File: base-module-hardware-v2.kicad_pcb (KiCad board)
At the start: 4 copper layers, 99.7 x 99.7 mm, 270 parts, among them K1 CONN_3, P1 PINBALL-CONNECTOR, P2 PINBALL-CONNECTOR, P3 SOLENOID-CONNECTOR, P4 CONN_16, P5 CONN_16, P6 HE10-34, Q1 BC846, Q10 DMN6040SSD, Q11 BC846, Q12 BC846, Q13 DMP2240UDM, Q14 DMP2240UDM, Q15 BC846, Q16 BC846, Q17 BC846, Q18 BC846, Q19 DMN6040SSD, Q2 BC846, Q20 DMN6040SSD, Q21 BC846, Q22 BC846, Q23 BC846, Q24 BC846, Q25 BC846, Q26 BC846, Q27 BC846, Q28 BC846, Q3 DMN6040SSD, Q30 FDD5614P, Q31 BC846, Q32 BSS138, Q4 DMN6040SSD, Q5 BC846, Q6 BC846, Q7 BC846, Q8 BC846, Q9 DMN6040SSD, U1 74LVC14, U2 STM32F072R, U3 MCP2562, U4 MC78L05, U5 AP1117IE33G, U6 ZXCT1086E5TA, U7 ZXCT1107SA-7, U8 LM7805CT, U9 MMA8653FC, X1 8.000 MHz

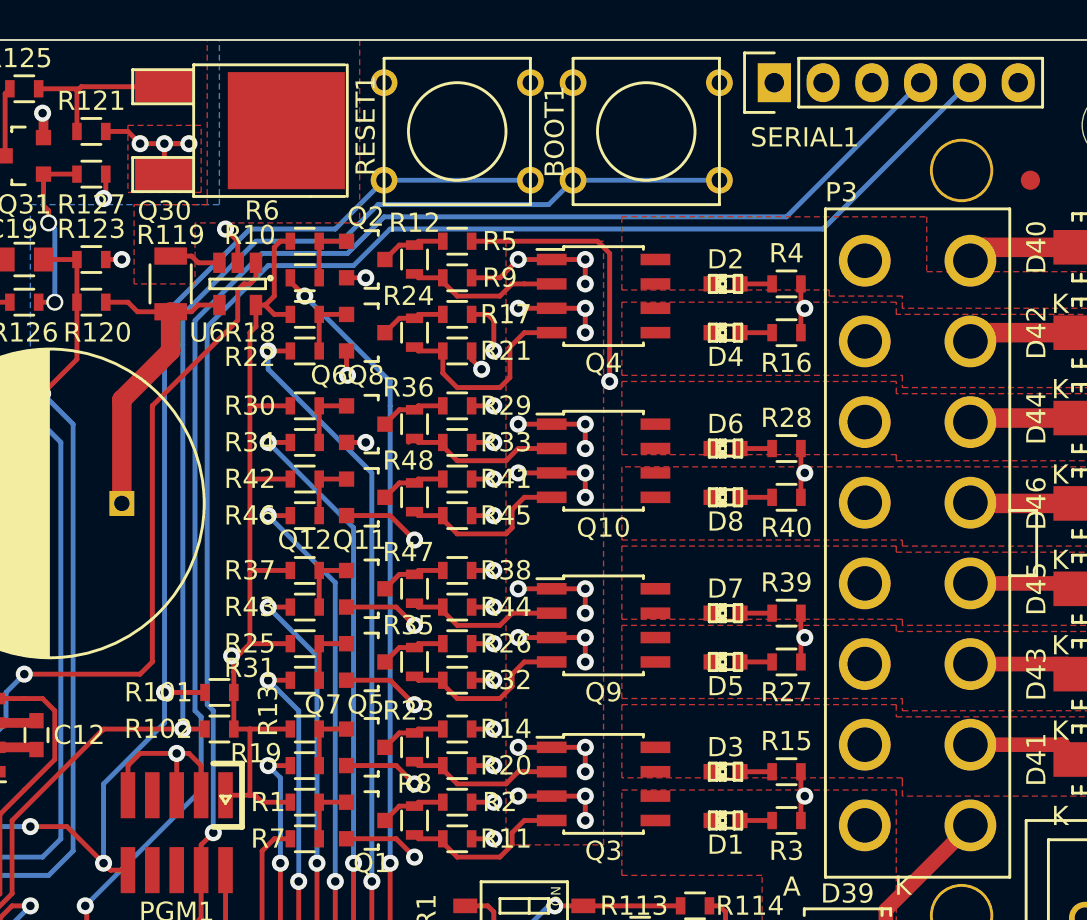
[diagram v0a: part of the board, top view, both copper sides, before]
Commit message: Latest changes (so old I don't remember)
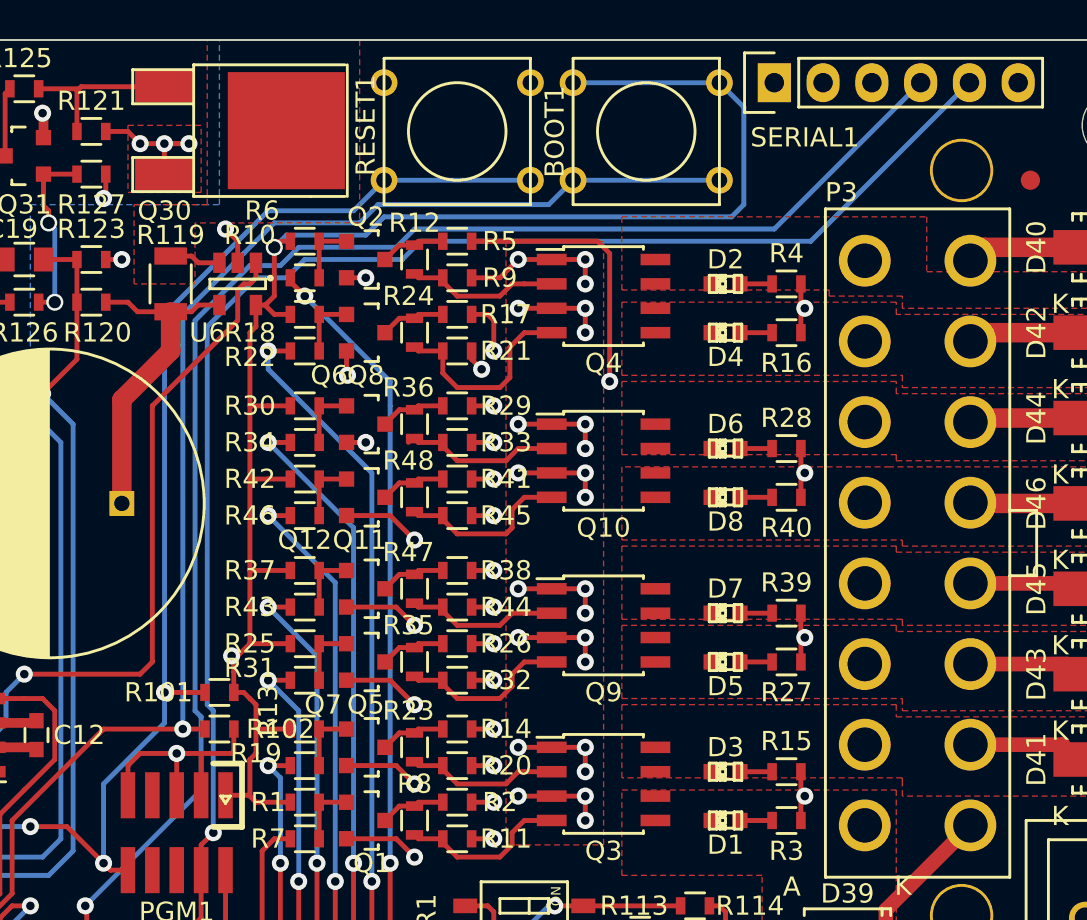
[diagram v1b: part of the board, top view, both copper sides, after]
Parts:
- turned BOOT1 to 180 degrees
- turned R102 to 0 degrees
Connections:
- BOOT1 pad 1: GND -> /Control Logic/BOOTLOADER
- BOOT1 pad 2: /Control Logic/BOOTLOADER -> +3.3V
- R102 pad 1: +3.3V -> /Control Logic/BOOTLOADER
- R102 pad 2: /Control Logic/BOOTLOADER -> GND
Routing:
- net +3.3V: track 211.6 -> 251.3 mm, vias 26 -> 27
- net GND: track 285.9 -> 289.2 mm
